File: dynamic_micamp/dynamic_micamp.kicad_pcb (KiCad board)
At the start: 2 copper layers, 72 x 47 mm, 20 parts, among them J1 AudioJack3_123, J2 USB_B_Micro, J3 AudioJack3_123, U1 NJM4580

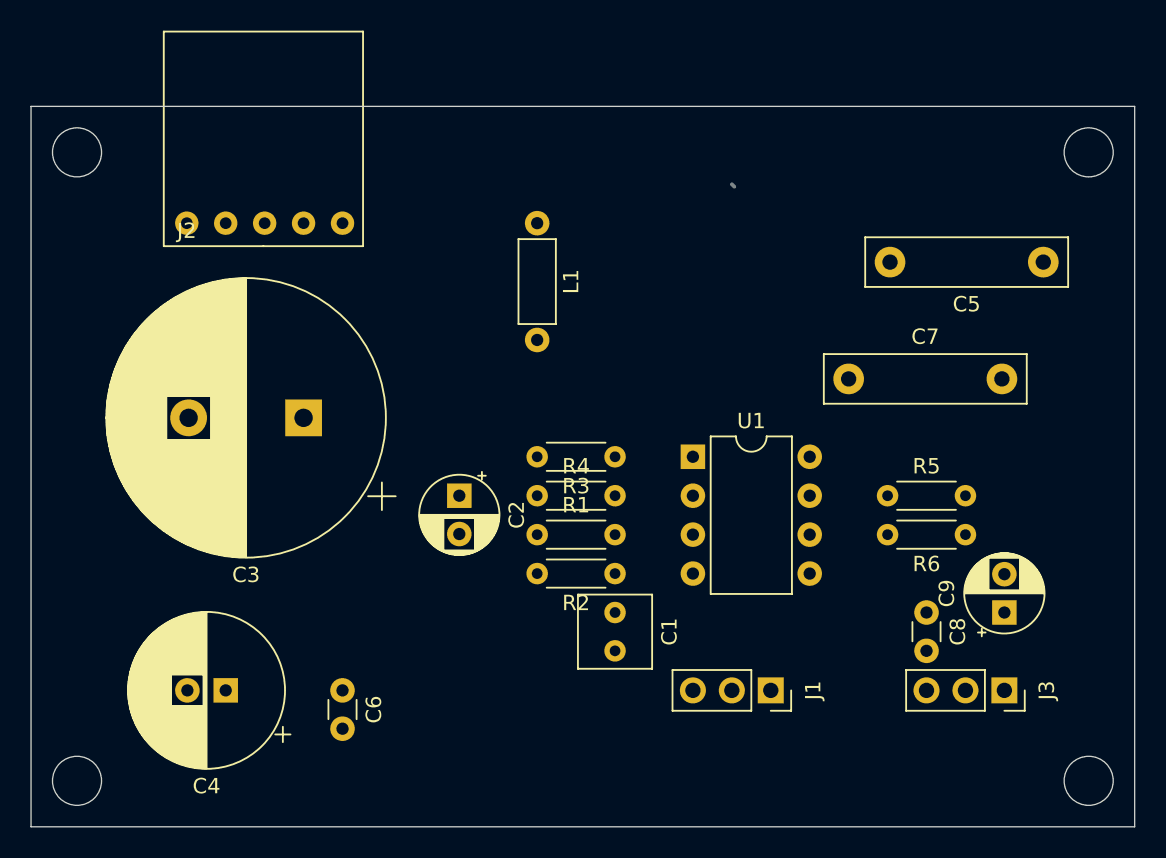
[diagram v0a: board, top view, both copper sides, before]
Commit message: done
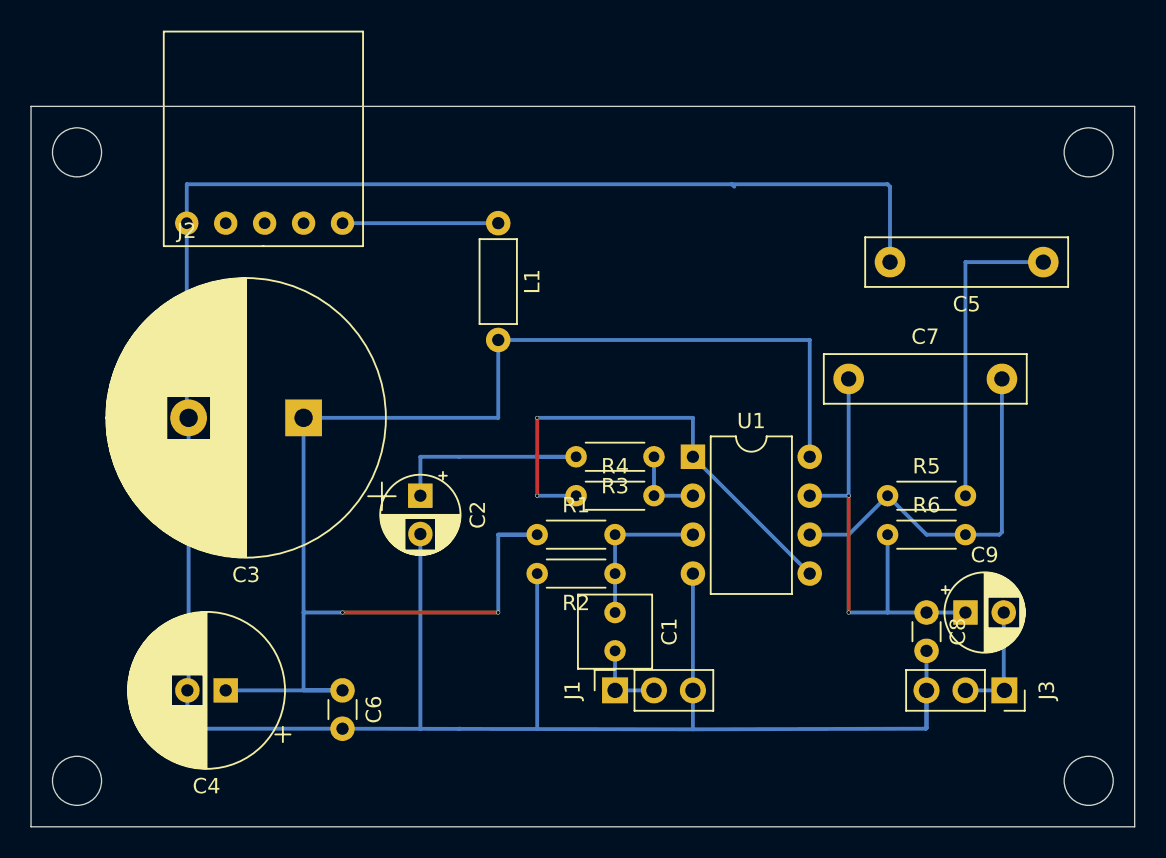
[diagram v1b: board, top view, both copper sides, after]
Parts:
- moved J1 10.2 mm to (68.1, 68.1), turned to 90 degrees
- moved R6 5.08 mm to (85.9, 57.9), turned to 0 degrees
- moved C9 2.54 mm to (91.0, 63.0), turned to 0 degrees
- moved L1 2.54 mm to (60.5, 37.6)
- moved R3 2.54 mm to (70.6, 52.9)
- moved C2 2.54 mm to (55.4, 55.4)
- moved R4 2.54 mm to (65.6, 55.4)
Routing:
- net GND: track 0.34 -> 175.6 mm
- net VCC: track 0.00 -> 96.5 mm, vias 0 -> 2
- net Net-(R4-Pad1): track 0.00 -> 31.1 mm, vias 0 -> 2
- net Net-(C7-Pad1): track 0.00 -> 30.5 mm, vias 0 -> 2
- net Net-(C7-Pad2): track 0.00 -> 24.7 mm
- net Net-(C5-Pad1): track 0.00 -> 20.3 mm
- net Net-(C2-Pad1): track 0.00 -> 15.2 mm
- net Net-(C1-Pad1): track 0.00 -> 10.2 mm
- net Net-(J2-Pad1): track 0.00 -> 10.2 mm
- net Net-(C9-Pad2): track 0.00 -> 7.64 mm
- net Net-(C1-Pad2): track 0.00 -> 5.12 mm
- net Net-(R3-Pad1): track 0.00 -> 5.08 mm
